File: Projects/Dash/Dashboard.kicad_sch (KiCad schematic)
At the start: 6 parts, among them J1 DTF13-6P, J2 Conn_01x03_Socket, J3 Conn_01x03_Socket, J4 Conn_01x03_Socket, U2 Adafruit-CAN-BFF-SMD

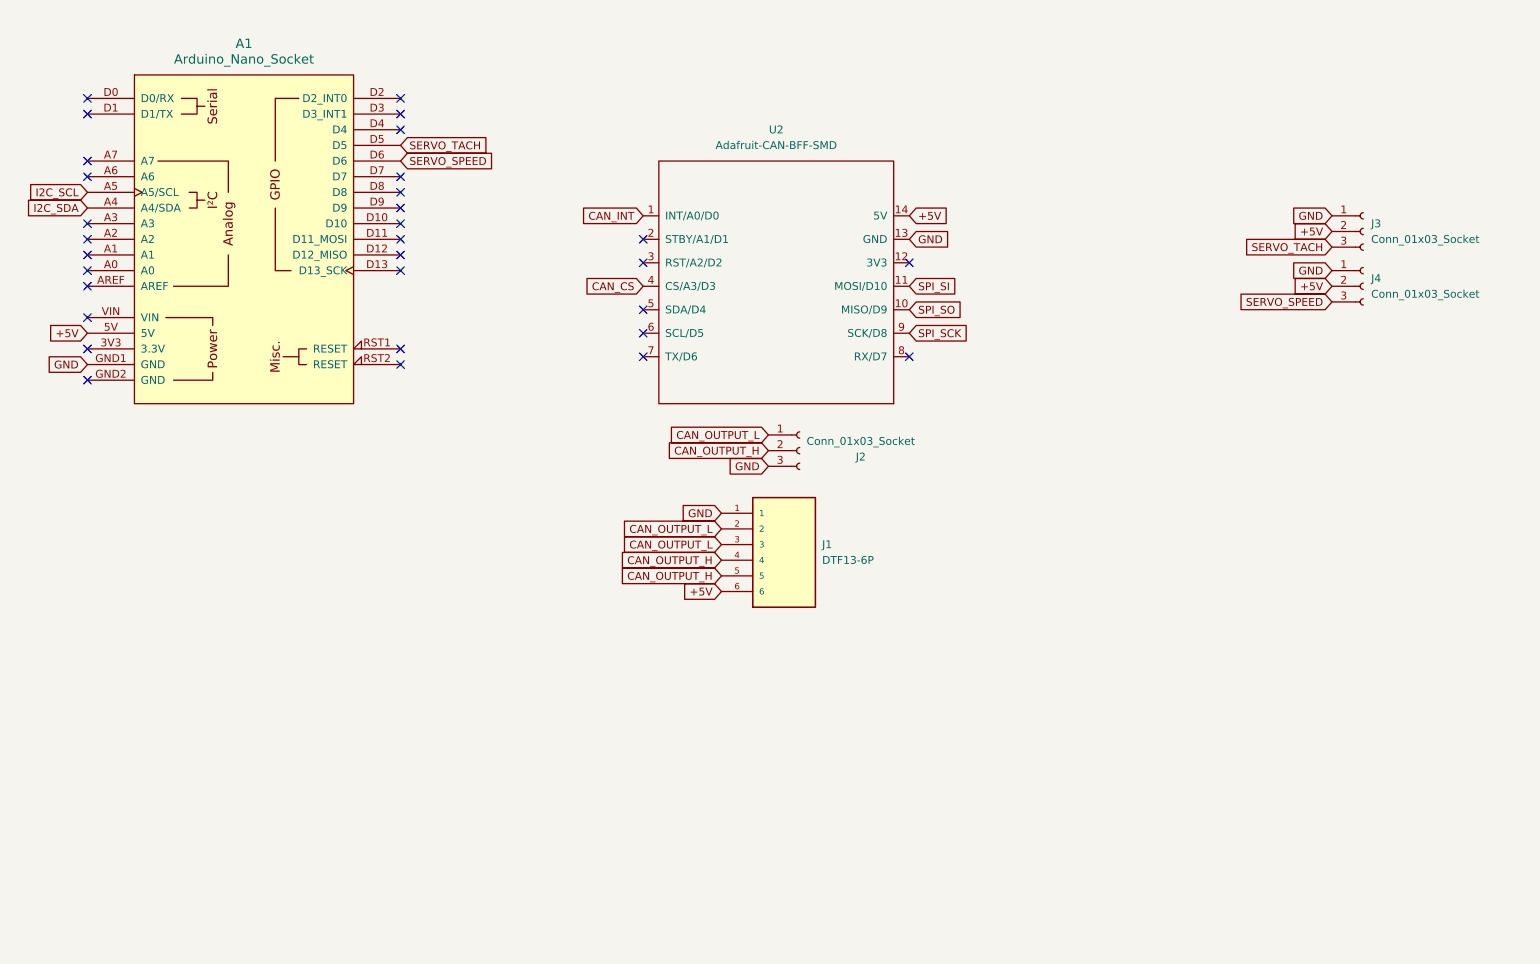
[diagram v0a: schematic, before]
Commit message: [2026-09-19] Dash REV 1 Done
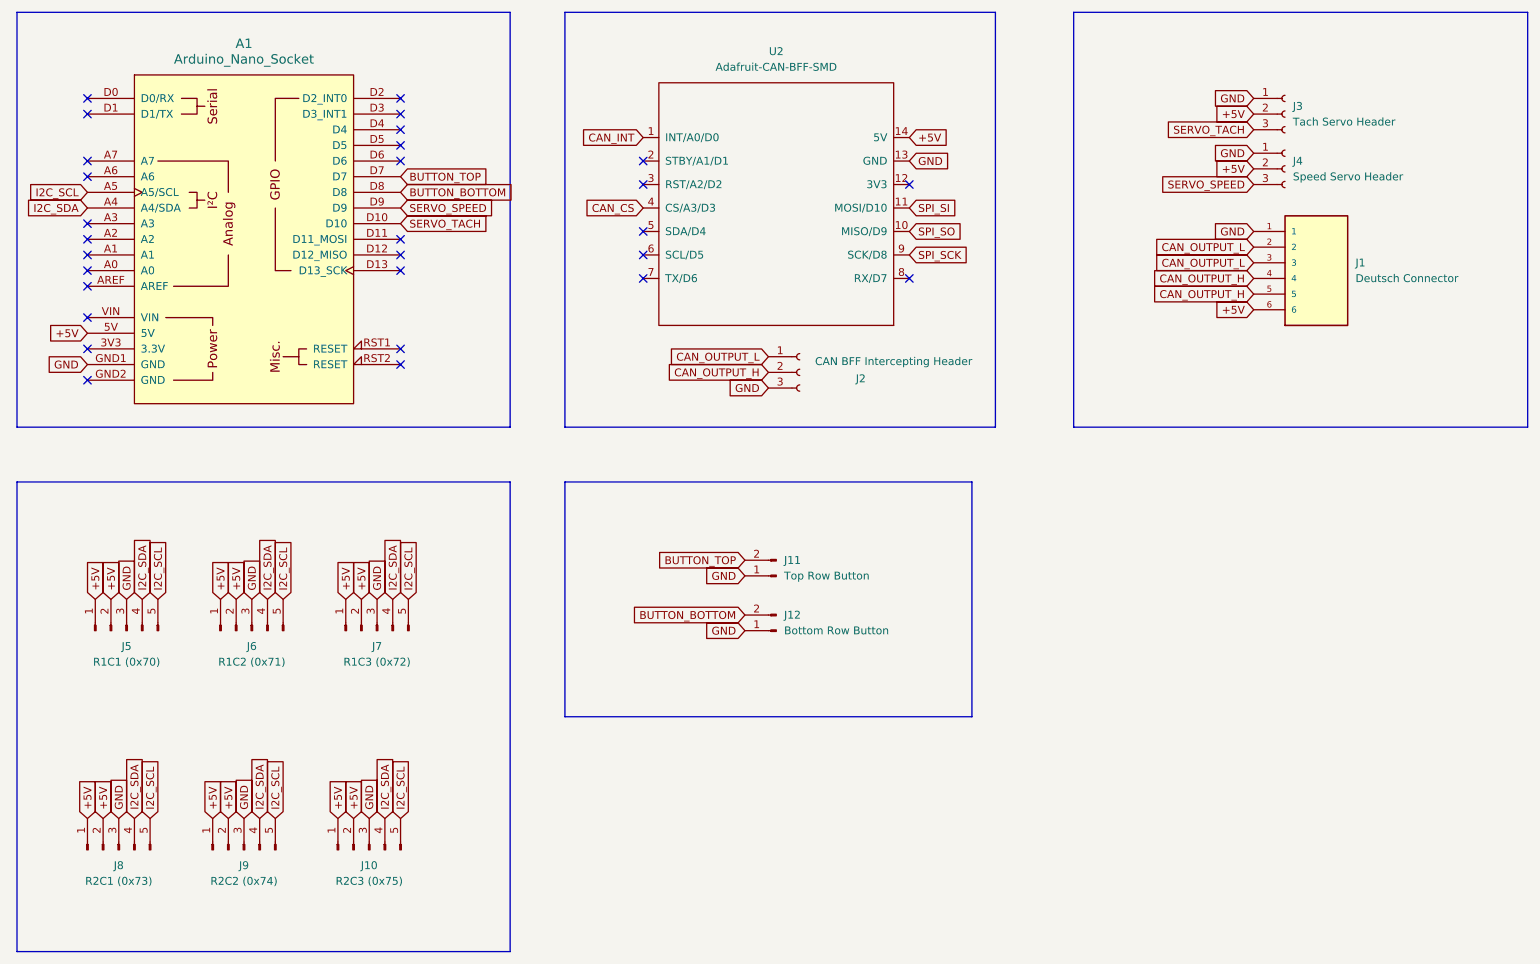
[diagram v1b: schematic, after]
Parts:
- added J10: R2C3 (0x75), Connector_PinHeader_2.54mm:PinHeader_1x05_P2.54mm_Vertical, symbol Connector:Conn_01x05_Pin
- added J11: Top Row Button, Connector_PinHeader_2.54mm:PinHeader_1x02_P2.54mm_Vertical, symbol Connector:Conn_01x02_Pin
- added J12: Bottom Row Button, Connector_PinHeader_2.54mm:PinHeader_1x02_P2.54mm_Vertical, symbol Connector:Conn_01x02_Pin
- added J5: R1C1 (0x70), Connector_PinHeader_2.54mm:PinHeader_1x05_P2.54mm_Vertical, symbol Connector:Conn_01x05_Pin
- added J6: R1C2 (0x71), Connector_PinHeader_2.54mm:PinHeader_1x05_P2.54mm_Vertical, symbol Connector:Conn_01x05_Pin
- added J7: R1C3 (0x72), Connector_PinHeader_2.54mm:PinHeader_1x05_P2.54mm_Vertical, symbol Connector:Conn_01x05_Pin
- added J8: R2C1 (0x73), Connector_PinHeader_2.54mm:PinHeader_1x05_P2.54mm_Vertical, symbol Connector:Conn_01x05_Pin
- added J9: R2C2 (0x74), Connector_PinHeader_2.54mm:PinHeader_1x05_P2.54mm_Vertical, symbol Connector:Conn_01x05_Pin
- J1: value DTF13-6P -> Deutsch Connector
- J2: value Conn_01x03_Socket -> CAN BFF Intercepting Header; footprint (none) -> Connector_PinHeader_2.54mm:PinHeader_1x03_P2.54mm_Vertical
- J3: value Conn_01x03_Socket -> Tach Servo Header; footprint (none) -> Connector_PinHeader_2.54mm:PinHeader_1x03_P2.54mm_Vertical
- J4: value Conn_01x03_Socket -> Speed Servo Header; footprint (none) -> Connector_PinHeader_2.54mm:PinHeader_1x03_P2.54mm_Vertical
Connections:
- net +5V: now also J10.1 (Pin_1), J10.2 (Pin_2), J5.1 (Pin_1), J5.2 (Pin_2), J6.1 (Pin_1), J6.2 (Pin_2), J7.1 (Pin_1), J7.2 (Pin_2), J8.1 (Pin_1), J8.2 (Pin_2), J9.1 (Pin_1), J9.2 (Pin_2)
- net GND: now also J10.3 (Pin_3), J11.1 (Pin_1), J12.1 (Pin_1), J5.3 (Pin_3), J6.3 (Pin_3), J7.3 (Pin_3), J8.3 (Pin_3), J9.3 (Pin_3)
- net I2C_SCL: now also J10.5 (Pin_5), J5.5 (Pin_5), J6.5 (Pin_5), J7.5 (Pin_5), J8.5 (Pin_5), J9.5 (Pin_5)
- net I2C_SDA: now also J10.4 (Pin_4), J5.4 (Pin_4), J6.4 (Pin_4), J7.4 (Pin_4), J8.4 (Pin_4), J9.4 (Pin_4)
- net SERVO_SPEED: now also A1.D9; no longer A1.D6
- net SERVO_TACH: now also A1.D10; no longer A1.D5
- net BUTTON_TOP: now reaches A1.D7
- net BUTTON_TOP: now also J11.2 (Pin_2)
- net BUTTON_BOTTOM: now reaches A1.D8
- net BUTTON_BOTTOM: now also J12.2 (Pin_2)
- no-connect marks 31 -> 29
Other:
- moved on the sheet: J1, J2, J3, J4, U2

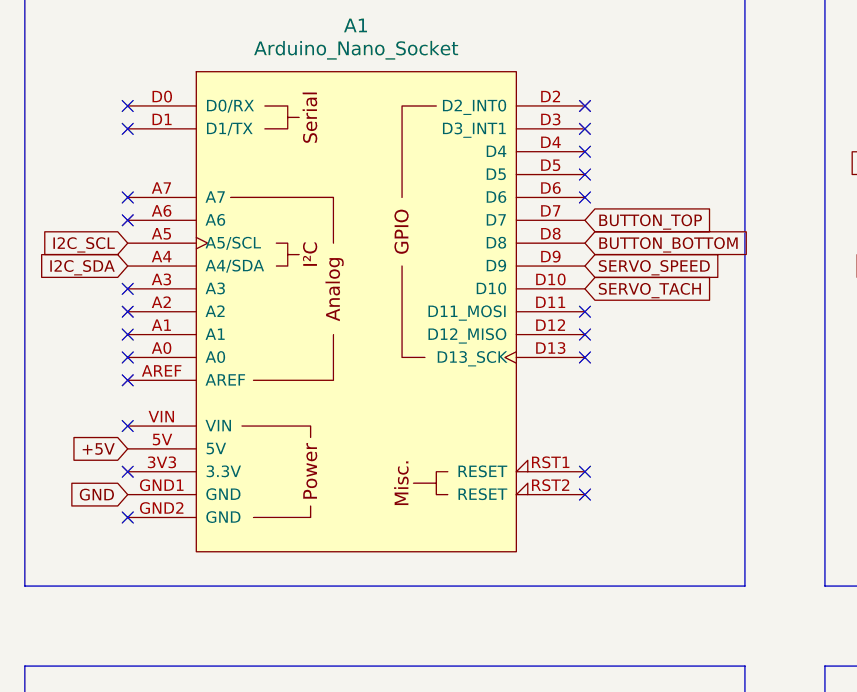
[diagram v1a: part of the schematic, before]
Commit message: Guess who forgot the SPI bus 😂
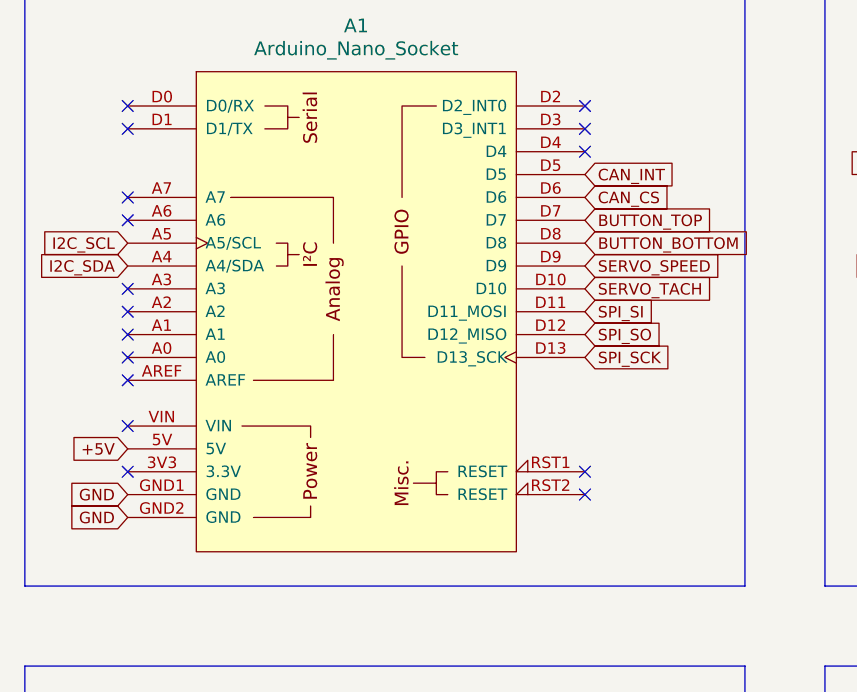
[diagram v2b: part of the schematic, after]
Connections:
- net CAN_CS: now also A1.D6
- net CAN_INT: now also A1.D5
- net GND: now also A1.GND2 (GND)
- net SPI_SCK: now also A1.D13 (D13_SCK)
- net SPI_SI: now also A1.D11 (D11_MOSI)
- net SPI_SO: now also A1.D12 (D12_MISO)
- no-connect marks 29 -> 23
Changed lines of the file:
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@@
-	)
-	(no_connect
-		(at 81.28 62.23)
-	)
-	(no_connect
-		(at 81.28 67.31)
 	)
 	(no_connect
@@
 	)
 	(no_connect
-		(at 81.28 49.53)
-	)
-	(no_connect
-		(at 81.28 64.77)
-	)
-	(no_connect
 		(at 30.48 39.37)
 	)
@@
 	)
 	(no_connect
-		(at 81.28 46.99)
-	)
-	(no_connect
 		(at 120.65 68.58)
 	)
@@
 	)
 	(no_connect
-		(at 30.48 85.09)
-	)
-	(no_connect
 		(at 30.48 59.69)
 	)
@@
 	(global_label "GND"
 		(shape input)
+		(at 30.48 85.09 180)
+		(fields_autoplaced yes)
+		(effects
+			(font
+				(size 1.27 1.27)
+			)
+			(justify right)
+		)
+		(property "Intersheetrefs" "${INTERSHEET_REFS}"
+			(at 23.6243 85.09 0)
+			(hide yes)
+			(show_name no)
+			(do_not_autoplace no)
+			(effects
+				(font
+					(size 1.27 1.27)
+				)
+				(justify right)
+			)
+		)
+	)
+	(global_label "GND"
+		(shape input)
 		(at 30.48 82.55 180)
 		(fields_autoplaced yes)
@@
 		)
 	)
+	(global_label "SPI_SCK"
+		(shape input)
+		(at 81.28 67.31 0)
+		(fields_autoplaced yes)
+		(effects
+			(font
+				(size 1.27 1.27)
+			)
+			(justify left)
+		)
+		(property "Intersheetrefs" "${INTERSHEET_REFS}"
+			(at 92.0666 67.31 0)
+			(hide yes)
+			(show_name no)
+			(do_not_autoplace no)
+			(effects
+				(font
+					(size 1.27 1.27)
+				)
+				(justify left)
+			)
+		)
+	)
 	(global_label "GND"
 		(shape input)
@@
 		)
 	)
+	(global_label "CAN_INT"
+		(shape input)
+		(at 81.28 46.99 0)
+		(fields_autoplaced yes)
+		(effects
+			(font
+				(size 1.27 1.27)
+			)
+			(justify left)
+		)
+		(property "Intersheetrefs" "${INTERSHEET_REFS}"
+			(at 91.8248 46.99 0)
+			(hide yes)
+			(show_name no)
+			(do_not_autoplace no)
+			(effects
+				(font
+					(size 1.27 1.27)
+				)
+				(justify left)
+			)
+		)
+	)
 	(global_label "I2C_SCL"
 		(shape input)
@@
 		)
 	)
+	(global_label "SPI_SI"
+		(shape input)
+		(at 81.28 62.23 0)
+		(fields_autoplaced yes)
+		(effects
+			(font
+				(size 1.27 1.27)
+			)
+			(justify left)
+		)
+		(property "Intersheetrefs" "${INTERSHEET_REFS}"
+			(at 90.1314 62.23 0)
+			(hide yes)
+			(show_name no)
+			(do_not_autoplace no)
+			(effects
+				(font
+					(size 1.27 1.27)
+				)
+				(justify left)
+			)
+		)
+	)
 	(global_label "SERVO_TACH"
 		(shape input)
@@
 		)
 	)
+	(global_label "CAN_CS"
+		(shape input)
+		(at 81.28 49.53 0)
+		(fields_autoplaced yes)
+		(effects
+			(font
+				(size 1.27 1.27)
+			)
+			(justify left)
+		)
+		(property "Intersheetrefs" "${INTERSHEET_REFS}"
+			(at 91.4014 49.53 0)
+			(hide yes)
+			(show_name no)
+			(do_not_autoplace no)
+			(effects
+				(font
+					(size 1.27 1.27)
+				)
+				(justify left)
+			)
+		)
+	)
 	(global_label "+5V"
 		(shape input)
@@
 			)
 		)
+	)
+	(global_label "SPI_SO"
+		(shape input)
+		(at 81.28 64.77 0)
+		(fields_autoplaced yes)
+		(effects
+			(font
+				(size 1.27 1.27)
+			)
+			(justify left)
+		)
+		(property "Intersheetrefs" "${INTERSHEET_REFS}"
+			(at 90.8571 64.77 0)
+			(hide yes)
+			(show_name no)
+			(do_not_autoplace no)
+			(effects
+				(font
+					(size 1.27 1.27)
+				)
+				(justify left)
+			)
+		)
